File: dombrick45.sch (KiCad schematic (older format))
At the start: 24 parts, among them SW1 SW_Push, U1 ATmega32U4-AU, Y1 16MHz

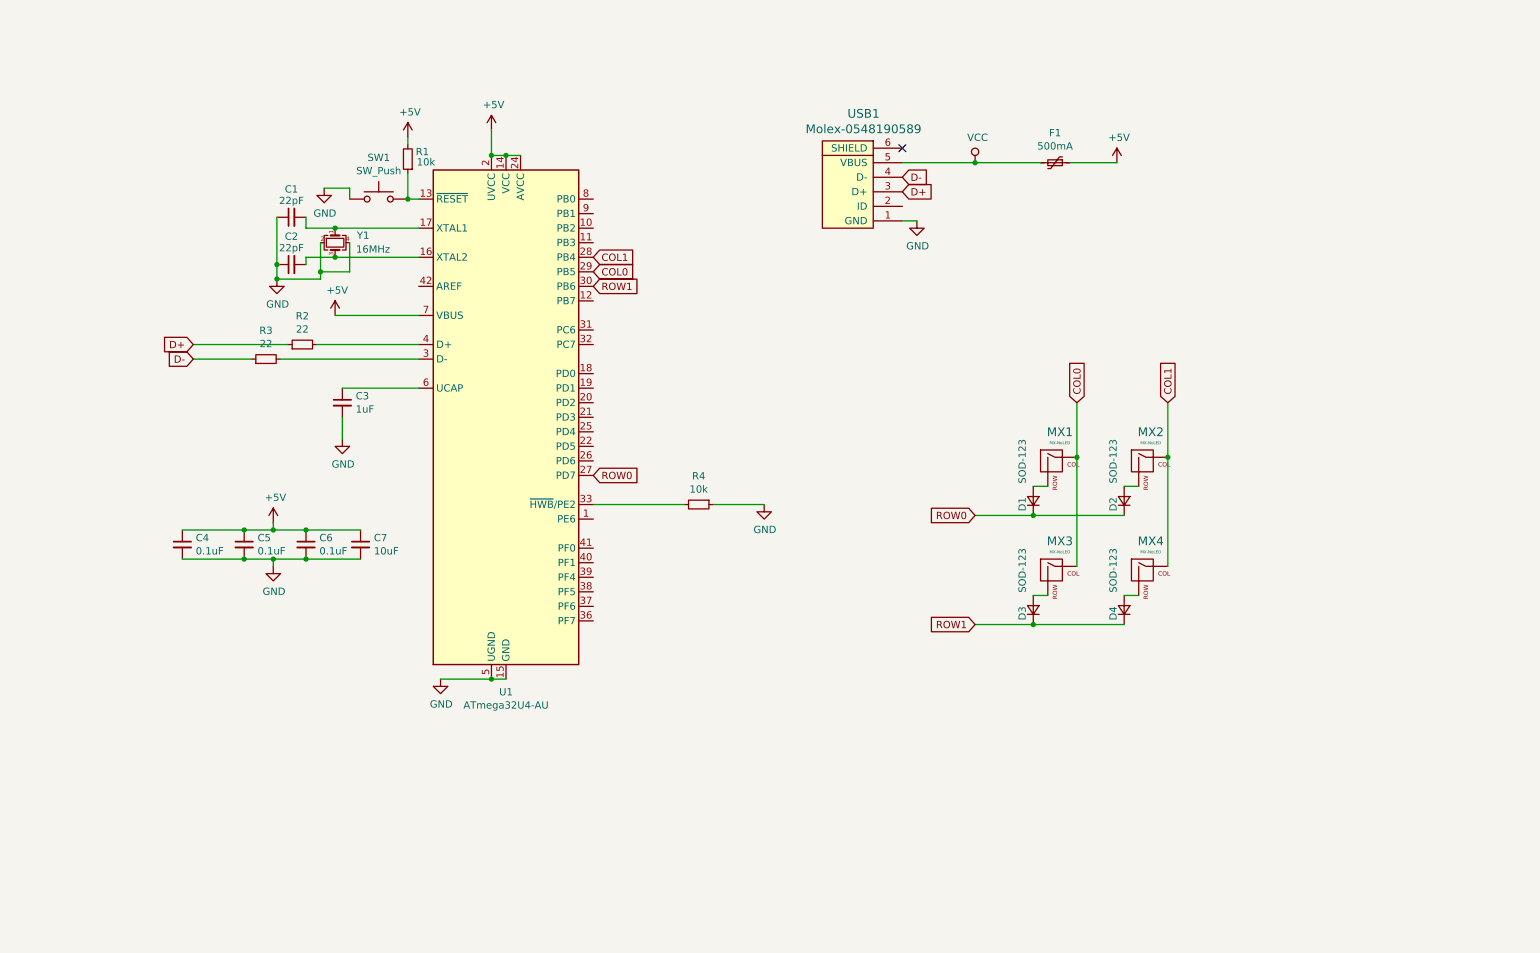
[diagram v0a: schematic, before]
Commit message: dombrick45 sematic to pcb tochuu
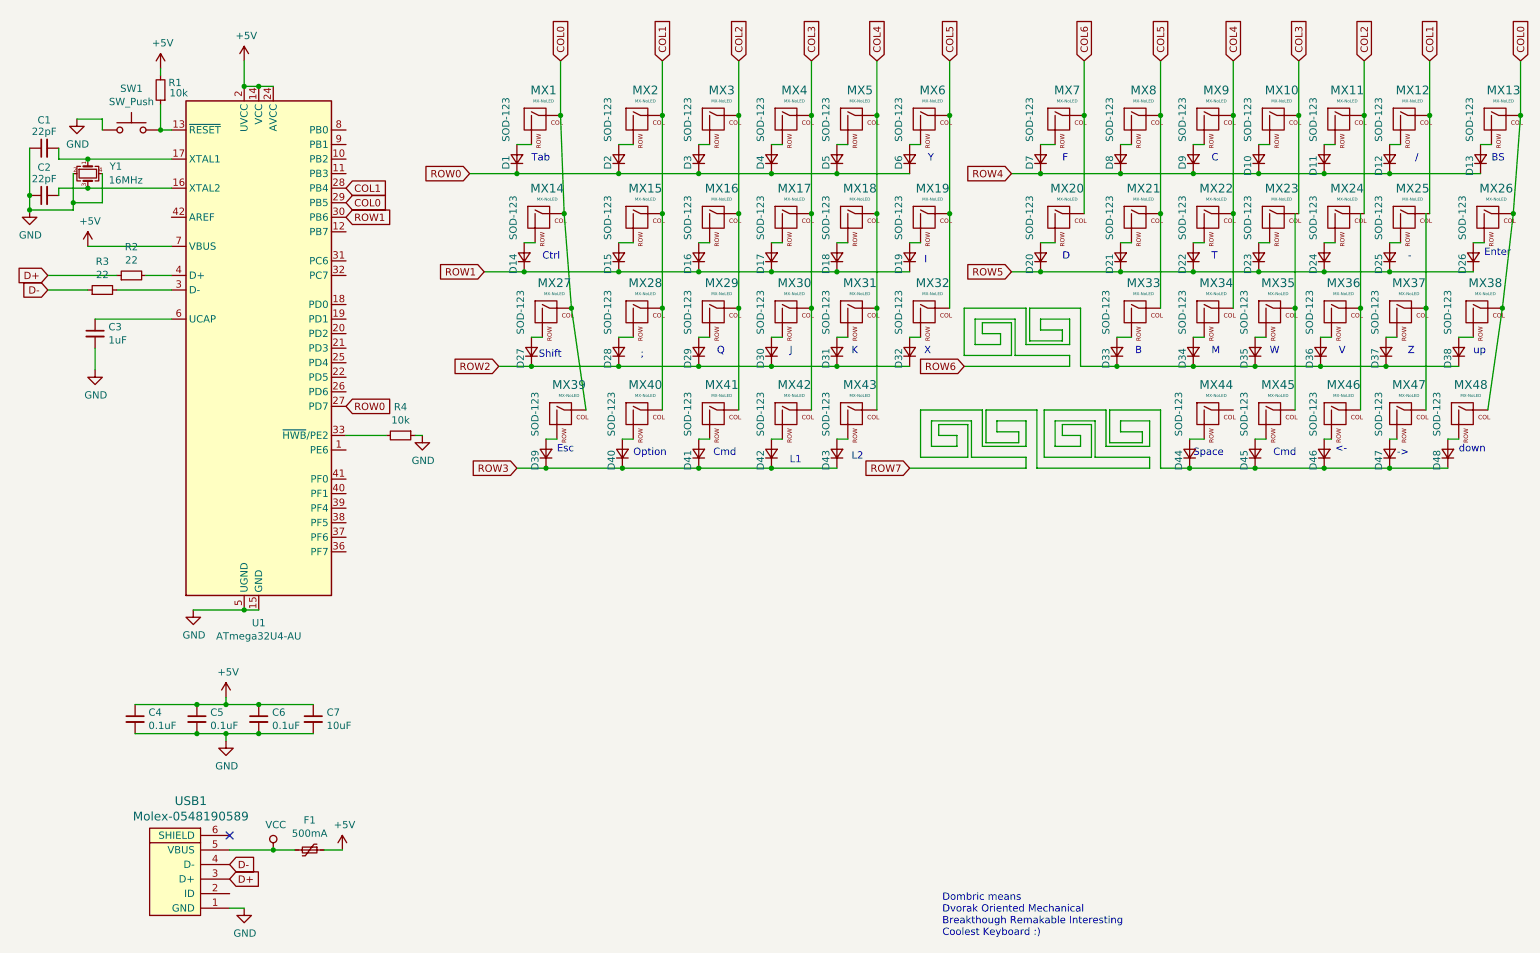
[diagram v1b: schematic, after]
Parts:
- added D10, D11, D12, D13, D16, D17, D18, D19, D20, D21, D22, D23, D24, D25, D26, D27, D28, D29, D3, D30, D31, D32, D33, D34, D35, D36, D37, D38, D39, D4, D40, D41, D42, D43, D44, D45, D46, D47, D48, D5, D6, D7, D8, D9: SOD-123, Diode_SMD:D_SOD-123, symbol Device:D_Small
- added MX10, MX11, MX12, MX16, MX17, MX18, MX19, MX20, MX21, MX22, MX23, MX24, MX25, MX26, MX28, MX29, MX3, MX30, MX31, MX32, MX33, MX34, MX35, MX36, MX37, MX38, MX39, MX4, MX40, MX46, MX47, MX48, MX5, MX6, MX7, MX8, MX9: MX-NoLED, MX_Alps_Hybrid:MX-1U-NoLED, symbol MX_Alps_Hybrid:MX-NoLED
- added MX13, MX27, MX41, MX42, MX43, MX45: MX-NoLED, MX_Alps_Hybrid:MX-1.25U-NoLED, symbol MX_Alps_Hybrid:MX-NoLED
- added MX44: MX-NoLED, MX_Alps_Hybrid:MX-2.75U-NoLED, symbol MX_Alps_Hybrid:MX-NoLED
- MX14: renamed from MX3; footprint MX_Alps_Hybrid:MX-1U-NoLED -> MX_Alps_Hybrid:MX-1.25U-NoLED
- renumbered D3 to D14, D4 to D15, MX4 to MX15
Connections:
- net COL0: now also MX13.1 (COL), MX26.1 (COL), MX27.1 (COL), MX38.1 (COL), MX39.1 (COL), MX48.1 (COL)
- net COL1: now also MX12.1 (COL), MX25.1 (COL), MX28.1 (COL), MX40.1 (COL)
- net ROW0: now also D3.1 (K), D4.1 (K), D5.1 (K), D6.1 (K)
- net ROW1: now also D16.1 (K), D17.1 (K), D18.1 (K), D19.1 (K)
- new net: D3.2 (A), MX3.2 (ROW)
- new net: D4.2 (A), MX4.2 (ROW)
- new net: D5.2 (A), MX5.2 (ROW)
- new net: D6.2 (A), MX6.2 (ROW)
- new net: D16.2 (A), MX16.2 (ROW)
- new net: D17.2 (A), MX17.2 (ROW)
- new net: D18.2 (A), MX18.2 (ROW)
- new net: D19.2 (A), MX19.2 (ROW)
- new net: D28.2 (A), MX28.2 (ROW)
- new net: D27.2 (A), MX27.2 (ROW)
- new net: D29.2 (A), MX29.2 (ROW)
- new net: D30.2 (A), MX30.2 (ROW)
- new net: D31.2 (A), MX31.2 (ROW)
- new net: D32.2 (A), MX32.2 (ROW)
- new net: D39.2 (A), MX39.2 (ROW)
- new net: D40.2 (A), MX40.2 (ROW)
- new net: D41.2 (A), MX41.2 (ROW)
- new net: D42.2 (A), MX42.2 (ROW)
- new net: D43.2 (A), MX43.2 (ROW)
- new net: D7.2 (A), MX7.2 (ROW)
- new net: D20.2 (A), MX20.2 (ROW)
- new net: D8.2 (A), MX8.2 (ROW)
- new net: D9.2 (A), MX9.2 (ROW)
- new net: D10.2 (A), MX10.2 (ROW)
- new net: D11.2 (A), MX11.2 (ROW)
- new net: D21.2 (A), MX21.2 (ROW)
- new net: D22.2 (A), MX22.2 (ROW)
- new net: D23.2 (A), MX23.2 (ROW)
- new net: D24.2 (A), MX24.2 (ROW)
- new net: D33.2 (A), MX33.2 (ROW)
- new net: D34.2 (A), MX34.2 (ROW)
- new net: MX35.1 (COL), MX45.1 (COL)
- new net: D35.2 (A), MX35.2 (ROW)
- new net: MX36.1 (COL), MX46.1 (COL)
- new net: D36.2 (A), MX36.2 (ROW)
- new net: MX37.1 (COL), MX47.1 (COL)
- new net: D37.2 (A), MX37.2 (ROW)
- new net: D44.2 (A), MX44.2 (ROW)
- new net: D45.2 (A), MX45.2 (ROW)
- new net: D46.2 (A), MX46.2 (ROW)
- new net: D47.2 (A), MX47.2 (ROW)
- new net: D48.2 (A), MX48.2 (ROW)
- new net: D12.2 (A), MX12.2 (ROW)
- new net: D25.2 (A), MX25.2 (ROW)
- new net: D38.2 (A), MX38.2 (ROW)
- new net: D13.2 (A), MX13.2 (ROW)
- new net: D26.2 (A), MX26.2 (ROW)
- new net COL2: MX11.1 (COL), MX16.1 (COL), MX24.1 (COL), MX29.1 (COL), MX3.1 (COL), MX41.1 (COL)
- new net COL3: MX10.1 (COL), MX17.1 (COL), MX23.1 (COL), MX30.1 (COL), MX4.1 (COL), MX42.1 (COL)
- new net COL4: MX18.1 (COL), MX22.1 (COL), MX31.1 (COL), MX34.1 (COL), MX43.1 (COL), MX5.1 (COL), MX9.1 (COL)
- new net COL5: MX19.1 (COL), MX21.1 (COL), MX32.1 (COL), MX33.1 (COL), MX6.1 (COL), MX8.1 (COL)
- new net COL6: MX20.1 (COL), MX7.1 (COL)
- new net ROW2: D27.1 (K), D28.1 (K), D29.1 (K), D30.1 (K), D31.1 (K), D32.1 (K)
- new net ROW3: D39.1 (K), D40.1 (K), D41.1 (K), D42.1 (K), D43.1 (K)
- new net ROW4: D10.1 (K), D11.1 (K), D12.1 (K), D13.1 (K), D7.1 (K), D8.1 (K), D9.1 (K)
- new net ROW5: D20.1 (K), D21.1 (K), D22.1 (K), D23.1 (K), D24.1 (K), D25.1 (K), D26.1 (K)
- new net ROW6: D33.1 (K), D34.1 (K), D35.1 (K), D36.1 (K), D37.1 (K), D38.1 (K)
- new net ROW7: D44.1 (K), D45.1 (K), D46.1 (K), D47.1 (K), D48.1 (K)
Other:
- note added: "-"
- note added: "->"
- note added: "/"
- note added: ";"
- note added: "<-"
- note added: "B"
- note added: "BS"
- note added: "C"
- note added: "Cmd"
- note added: "Ctrl"
- note added: "D"
- note added: "Dombric means \nDvorak Oriented Mechanical\nBreakthough Remakable Interesting\nCoolest Keyboard :)"
- note added: "Enter"
- note added: "Esc"
- note added: "F"
- note added: "I"
- note added: "J"
- note added: "K"
- note added: "L1"
- note added: "L2"
- note added: "M"
- note added: "Option"
- note added: "Q"
- note added: "Shift"
- note added: "Space"
- note added: "T"
- note added: "Tab"
- note added: "V"
- note added: "W"
- note added: "X"
- note added: "Y"
- note added: "Z"
- note added: "down"
- note added: "up"
- moved on the sheet: C1, C2, C3, C4, C5, C6, C7, D1, D14, D15, D2, F1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
